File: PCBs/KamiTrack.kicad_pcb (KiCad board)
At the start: 2 copper layers, 78.5 x 20.6 mm, 65 parts, among them J1 Conn_01x02_Female, J2 Conn_01x04_Female, J3 Conn_01x02_Female, J4 Conn_01x08_Female, J5 Conn_01x02_Female, P1 USB_C_Plug_USB2.0, SW1 Option/FLASH Switch, SW2 Cali Switch, SW3 SW_SPDT MAIN POWER, U1 ME6211C, U2 TP4056, U3 MPU-6050, U4 DW01, U5 FS8205A, U6 ESP-12F, U7 CH340C, U8 QMC5883L

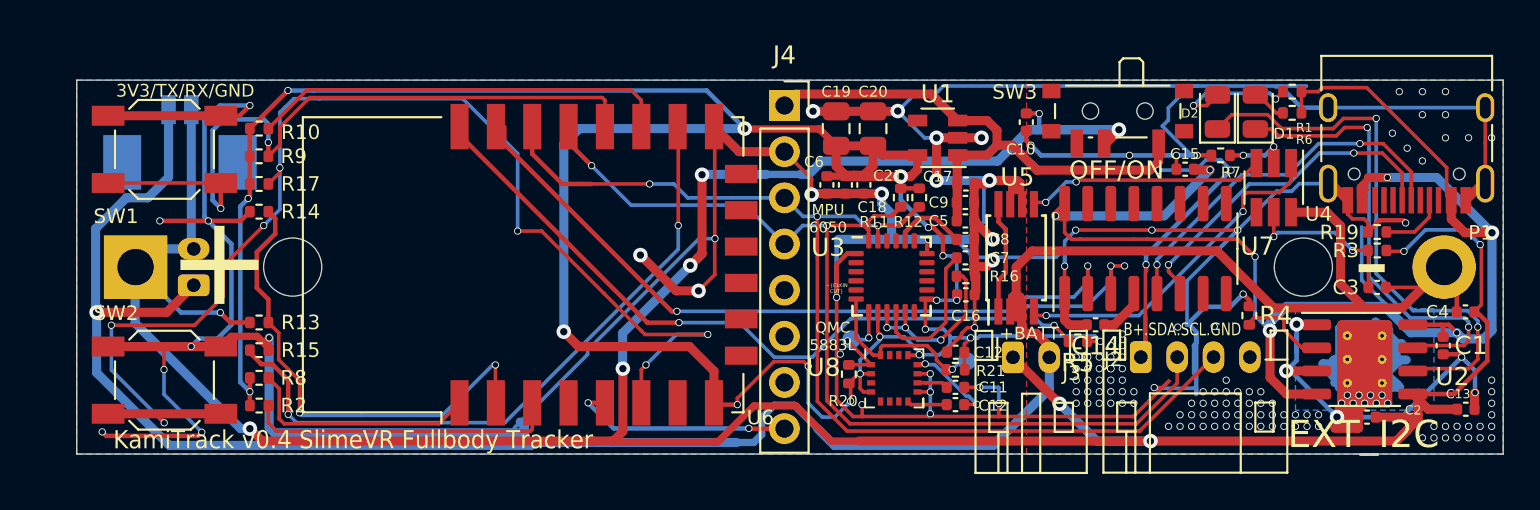
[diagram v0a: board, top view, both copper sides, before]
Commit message: add JLCPCB_CORRECTION
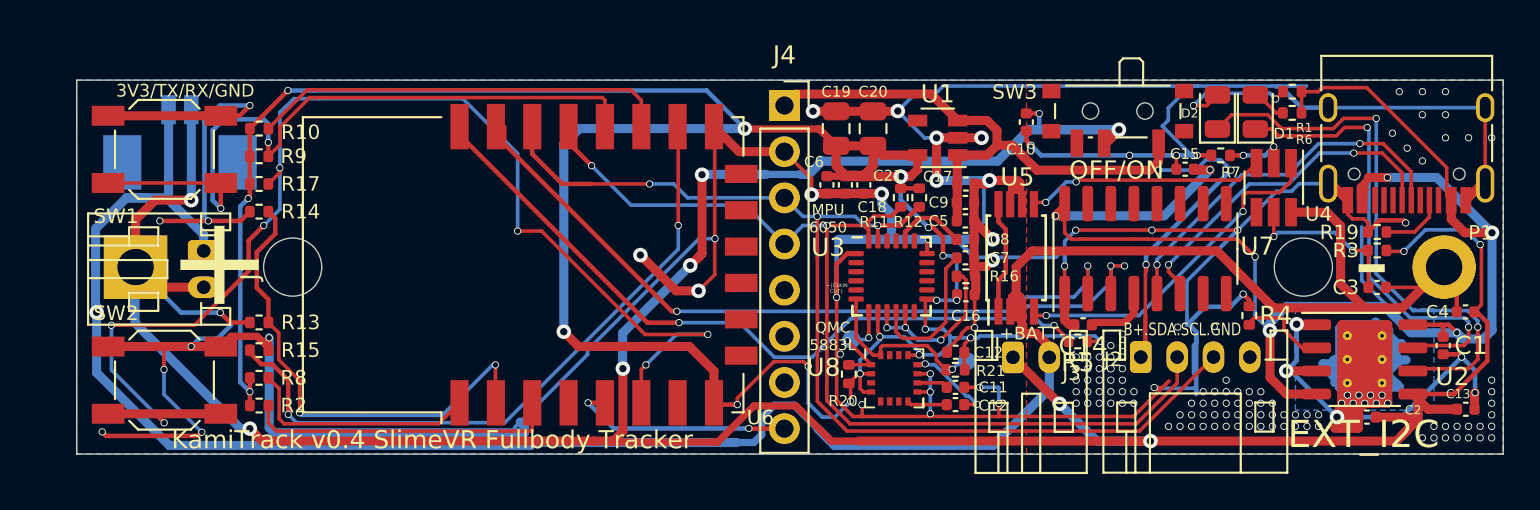
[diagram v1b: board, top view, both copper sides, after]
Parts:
- J1: footprint Connector_JST:JST_PH_B2B-PH-K_1x02_P2.00mm_Vertical -> Connector_JST:JST_PH_S2B-PH-K_1x02_P2.00mm_Horizontal; moved to F.Cu
- moved J1 1.97 mm to (96.8, 64.6), turned to -90 degrees
- moved C14 0.69 mm to (145.2, 68.7)
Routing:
- net GND: track 446.8 -> 439.6 mm
- net BATT+: track 185.2 -> 190.6 mm, vias 11 -> 12
- net Net-(C14-Pad1): track 3.26 -> 4.84 mm
